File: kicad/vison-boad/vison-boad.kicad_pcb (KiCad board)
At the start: 2 copper layers, 80 x 100 mm, 29 parts, among them J1 USB_C_Receptacle_USB2.0, J2 Wio Terminal, J3 UART, J4 pin_test, J5 NEO PIXEL, J6 to main, J7 I2C_0, SW1 BOOTSET, SW2 RESET, SW3 M1n_RST, U1 RP2040_Stamp, U2 M1n-break, U3 M1n-break, U4 M1n-break, U5 M1n-break, U6 M1n-break

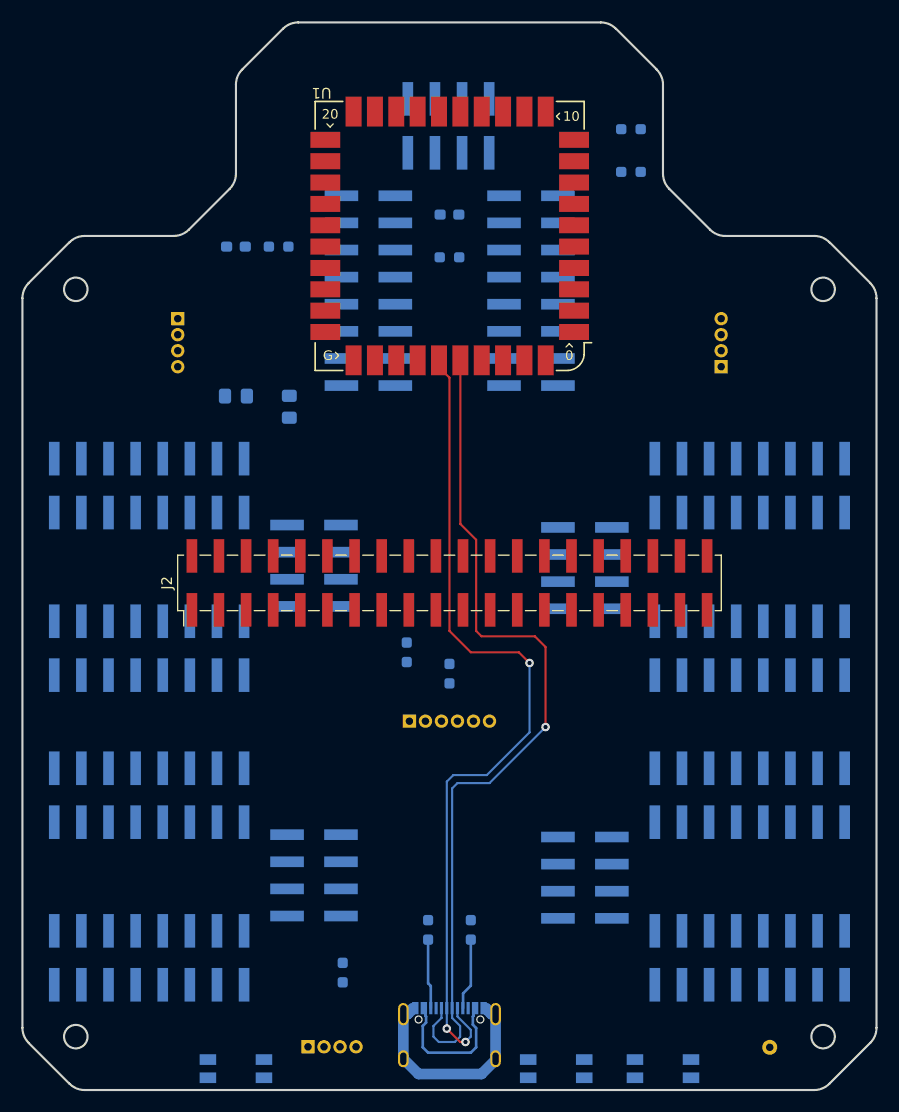
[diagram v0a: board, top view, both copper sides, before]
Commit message: fix: vison-board 配線後
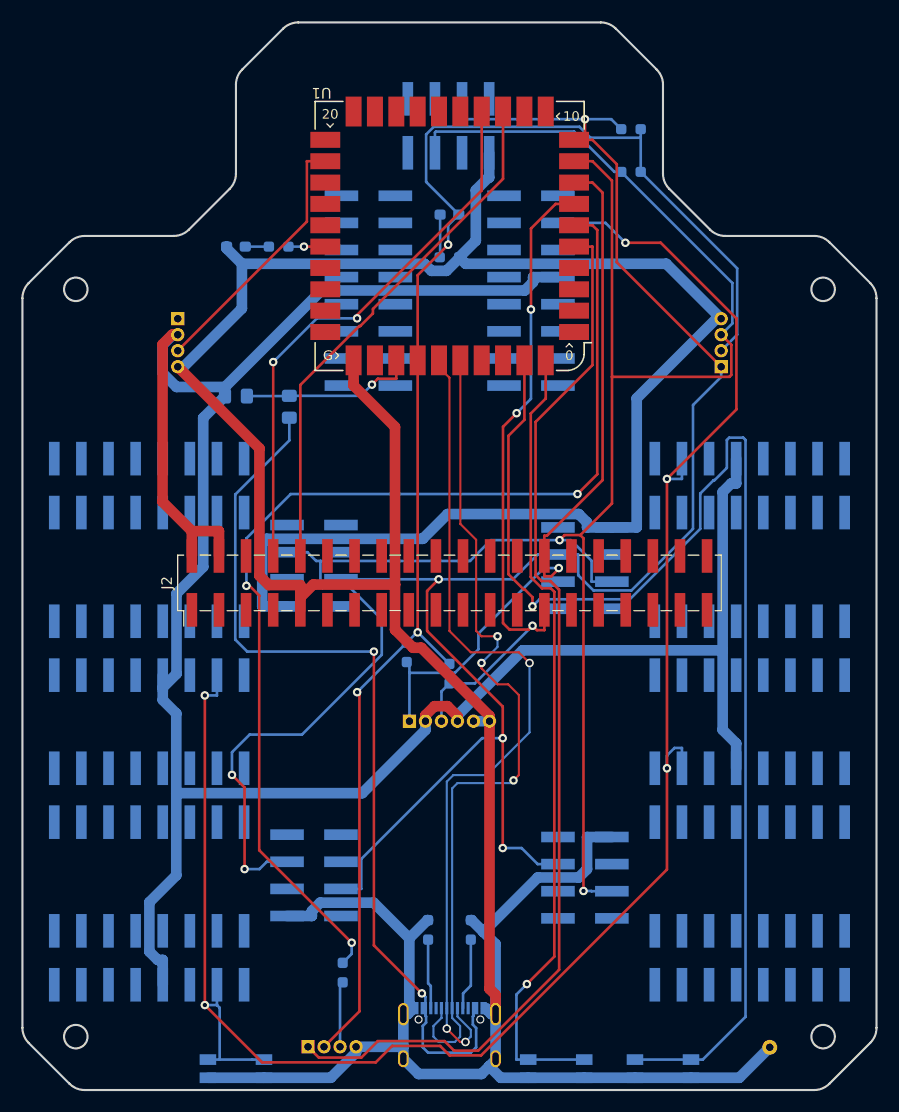
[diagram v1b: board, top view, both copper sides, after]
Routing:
- net GND: track 20.6 -> 368.0 mm
- net +5V: track 0.00 -> 225.7 mm
- net I2C_0.SDA: track 0.00 -> 213.9 mm, vias 0 -> 4
- net M1n_RST: track 0.00 -> 182.1 mm, vias 0 -> 5
- net I2C_0.SCL: track 0.00 -> 159.2 mm, vias 0 -> 4
- net +3.3V: track 0.00 -> 142.3 mm, vias 0 -> 3
- net /RESET: track 0.00 -> 120.8 mm, vias 0 -> 1
- net /RX_1: track 0.00 -> 105.0 mm, vias 0 -> 3
- net /TX_1: track 0.00 -> 101.1 mm
- net /BOOTSET: track 0.00 -> 75.3 mm, vias 0 -> 1
- net VBUS: track 13.6 -> 84.8 mm, vias 0 -> 2
- net I2C_1.SCL: track 0.00 -> 67.7 mm, vias 0 -> 1
- net I2C_1.SDA: track 0.00 -> 63.2 mm, vias 0 -> 3
- net /RX_0: track 0.00 -> 51.9 mm, vias 0 -> 2
- net /TX_0: track 0.00 -> 49.5 mm
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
